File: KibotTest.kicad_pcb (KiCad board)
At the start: 2 copper layers, 16 x 10.8 mm, 3 parts, among them J1 Conn_01x02

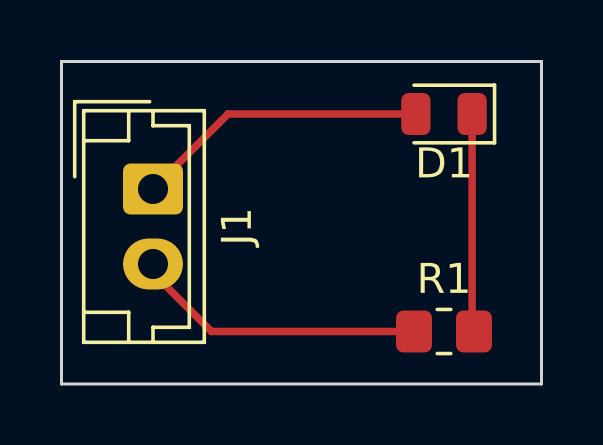
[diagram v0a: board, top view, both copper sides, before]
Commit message: [ACT] Test error detection
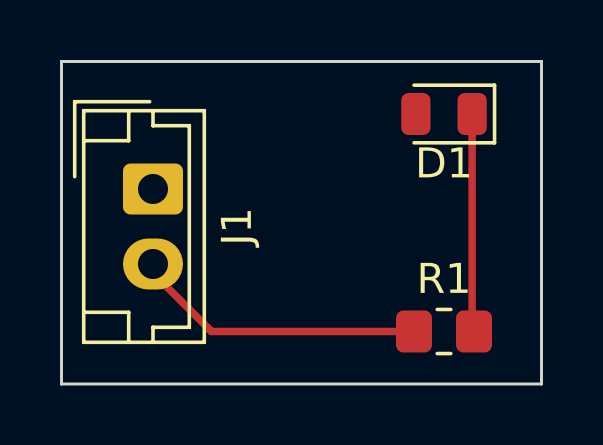
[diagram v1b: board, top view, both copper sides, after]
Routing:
- net +5V: track 9.80 -> 0.00 mm
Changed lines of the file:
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@@
   (segment (start 59.4375 52.9375) (end 59.5 53) (width 0.25) (layer "F.Cu") (net 1))
   (segment (start 59.4375 45.75) (end 59.4375 52.9375) (width 0.25) (layer "F.Cu") (net 1))
-  (segment (start 51.3 45.75) (end 48.8 48.25) (width 0.25) (layer "F.Cu") (net 2))
-  (segment (start 57.5625 45.75) (end 51.3 45.75) (width 0.25) (layer "F.Cu") (net 2))
   (segment (start 57.5 53) (end 50.75 53) (width 0.25) (layer "F.Cu") (net 3))
   (segment (start 48.8 51.05) (end 48.8 50.75) (width 0.25) (layer "F.Cu") (net 3))
